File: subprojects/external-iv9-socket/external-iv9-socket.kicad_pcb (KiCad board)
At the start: 2 copper layers, 17.8 x 16.3 mm, 3 parts, among them J1 PINHD_1x6_Male, J3 PINHD_1x4_Male

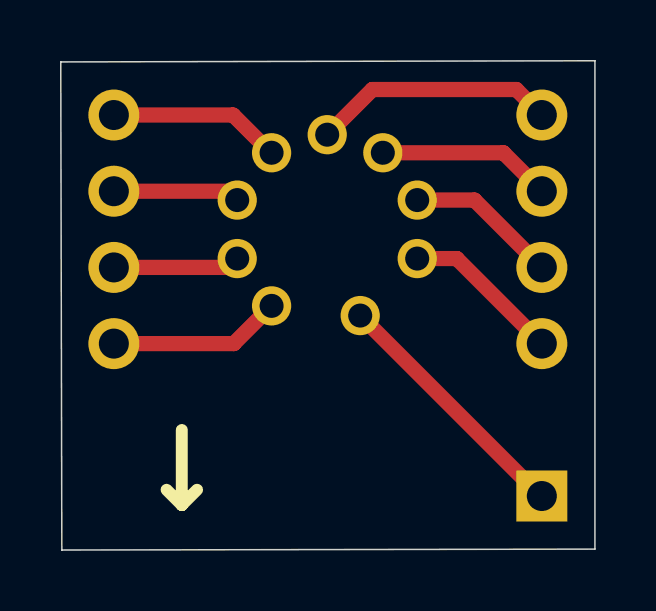
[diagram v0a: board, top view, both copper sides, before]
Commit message: Zase po dlhej dobe nejaký zálohovací commit.
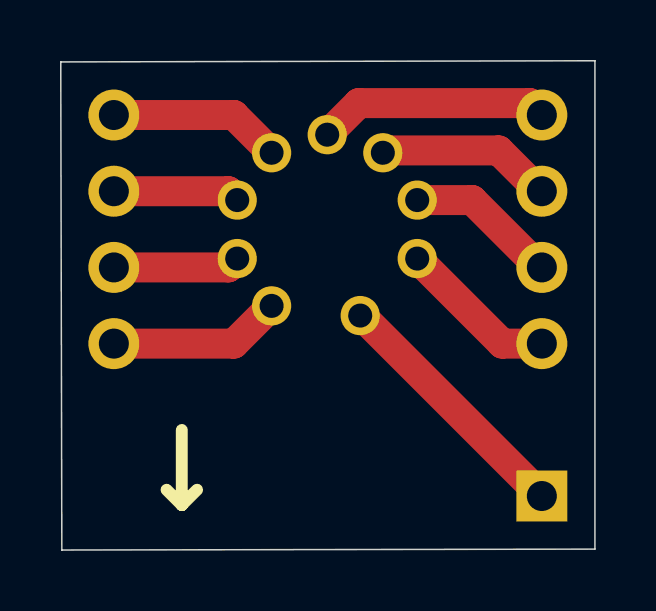
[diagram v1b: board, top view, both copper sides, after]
